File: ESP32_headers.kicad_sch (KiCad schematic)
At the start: 2 parts, among them J8 Conn_01x15_Socket, J9 Conn_01x15_Socket

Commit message: start compliance with PCBway
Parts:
- J8, J9: Item # (none) -> 11
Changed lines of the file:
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@@
+			)
+		)
+		(property "Item #" "11"
+			(at 58.42 59.69 0)
+			(effects
+				(font
+					(size 1.27 1.27)
+				)
+				(hide yes)
 			)
 		)
@@
 			(at 58.42 71.12 0)
 			(effects
+				(font
+					(size 1.27 1.27)
+				)
+				(hide yes)
+			)
+		)
+		(property "Item #" "11"
+			(at 58.42 71.12 0)
+			(effects

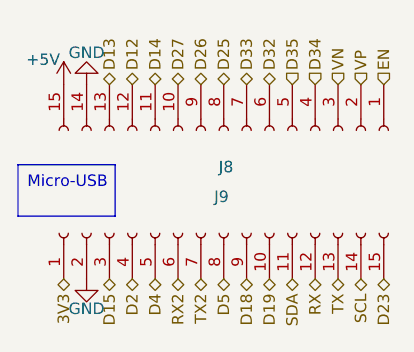
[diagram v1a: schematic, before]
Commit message: refresh stage 1
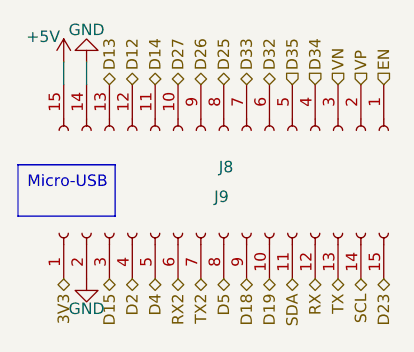
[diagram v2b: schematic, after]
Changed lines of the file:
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@@
 	(generator_version "8.0")
 	(paper "A4")
+	(wire
+		(pts
+			(xy 40.64 52.07) (xy 40.64 54.61)
+		)
+		(stroke
+			(width 0)
+			(type default)
+		)
+	)
+	(wire
+		(pts
+			(xy 43.18 52.07) (xy 43.18 54.61)
+		)
+		(stroke
+			(width 0)
+			(type default)
+		)
+	)
 	(text_box "Micro-USB"
 		(exclude_from_sim no)
@@
 	(symbol
 		(lib_id "power:GND")
-		(at 43.18 54.61 180)
+		(at 43.18 52.07 180)
 		(unit 1)
 		(exclude_from_sim no)
@@
 		(dnp no)
 		(property "Reference" "#PWR08"
-			(at 43.18 48.26 0)
+			(at 43.18 45.72 0)
 			(effects
 				(font
@@
 		)
 		(property "Value" "GND"
-			(at 43.18 51.054 0)
+			(at 43.18 48.514 0)
 			(effects
 				(font
@@
 		)
 		(property "Footprint" ""
-			(at 43.18 54.61 0)
+			(at 43.18 52.07 0)
 			(effects
 				(font
@@
 		)
 		(property "Datasheet" ""
-			(at 43.18 54.61 0)
+			(at 43.18 52.07 0)
 			(effects
 				(font
@@
 		)
 		(property "Description" "Power symbol creates a global label with name \"GND\" , ground"
-			(at 43.18 54.61 0)
+			(at 43.18 52.07 0)
 			(effects
 				(font
@@
 	(symbol
 		(lib_id "power:+5V")
-		(at 40.64 54.61 0)
+		(at 40.64 52.07 0)
 		(unit 1)
 		(exclude_from_sim no)
@@
 		(dnp no)
 		(property "Reference" "#PWR06"
-			(at 40.64 58.42 0)
+			(at 40.64 55.88 0)
 			(effects
 				(font
@@
 		)
 		(property "Value" "+5V"
-			(at 38.354 51.816 0)
+			(at 38.354 49.276 0)
 			(effects
 				(font
@@
 		)
 		(property "Footprint" ""
-			(at 40.64 54.61 0)
+			(at 40.64 52.07 0)
 			(effects
 				(font
@@
 		)
 		(property "Datasheet" ""
-			(at 40.64 54.61 0)
+			(at 40.64 52.07 0)
 			(effects
 				(font
@@
 		)
 		(property "Description" "Power symbol creates a global label with name \"+5V\""
-			(at 40.64 54.61 0)
-			(effects
-				(font
+			(at 40.64 52.07 0)
+			(effects
+				(font
